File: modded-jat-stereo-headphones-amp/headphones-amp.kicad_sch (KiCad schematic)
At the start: 52 parts, among them J1 9V-15V, J2 9V-15V, J3 Input, J4 Headphones out, Q1 BD139, Q2 BD140, Q3 BD139, Q4 BD140, SW1 POWER ON, U1 NE5532

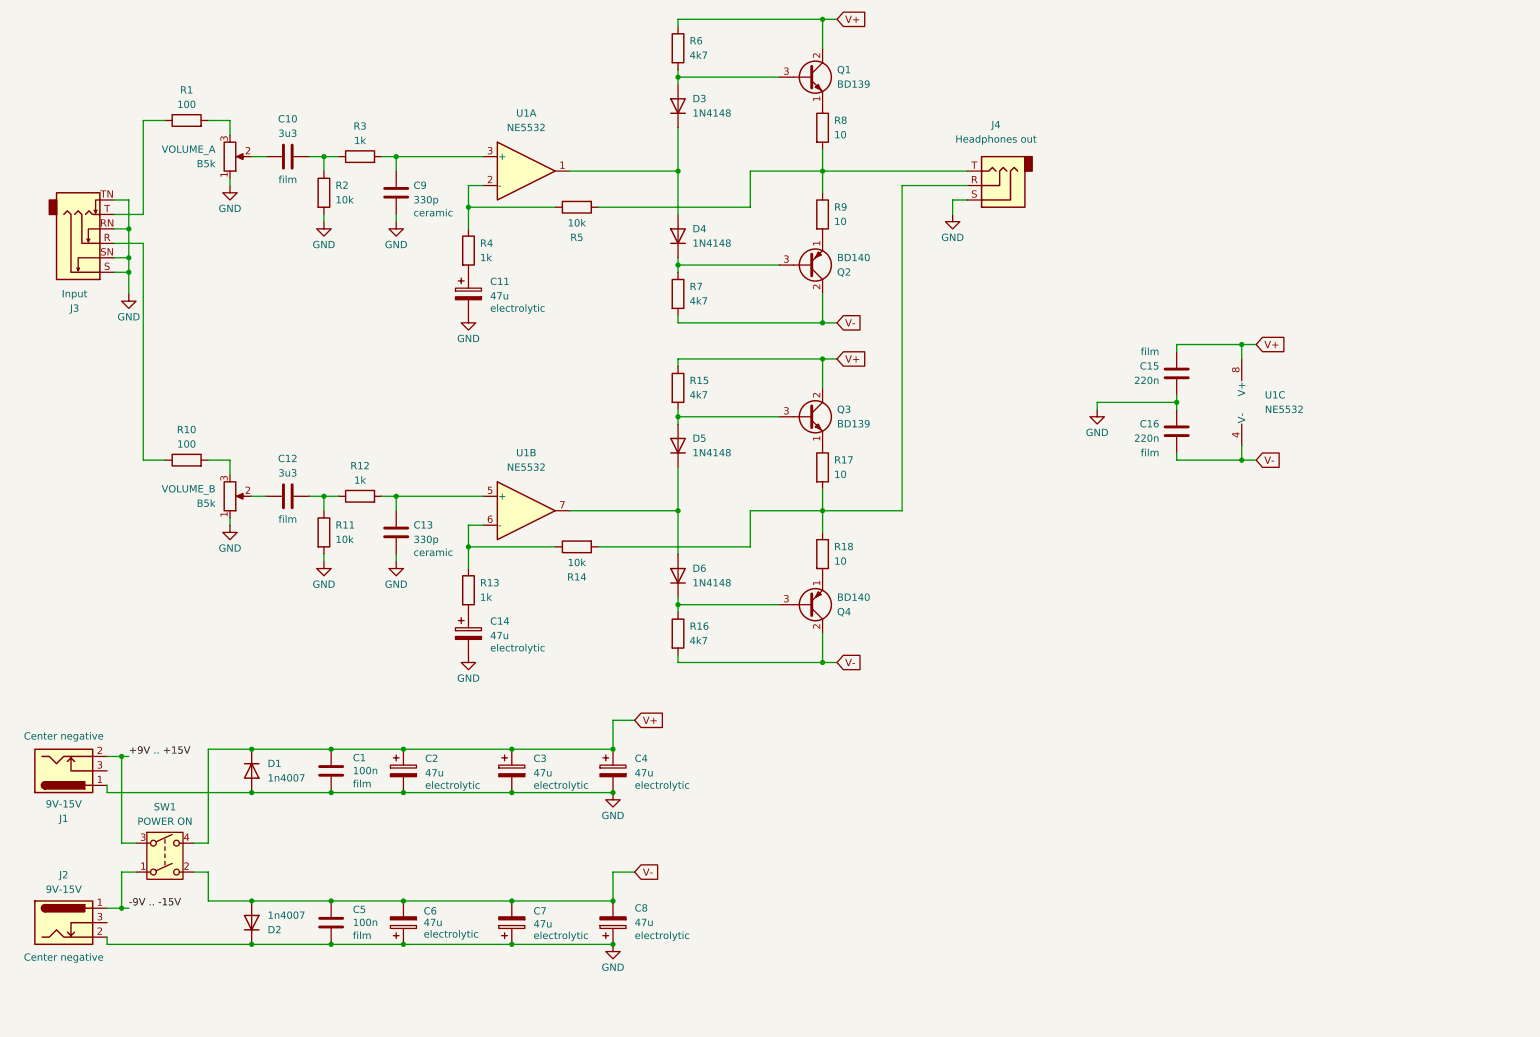
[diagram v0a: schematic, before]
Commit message: modded-jat-stereo-headphones-amp: r2-wip-1
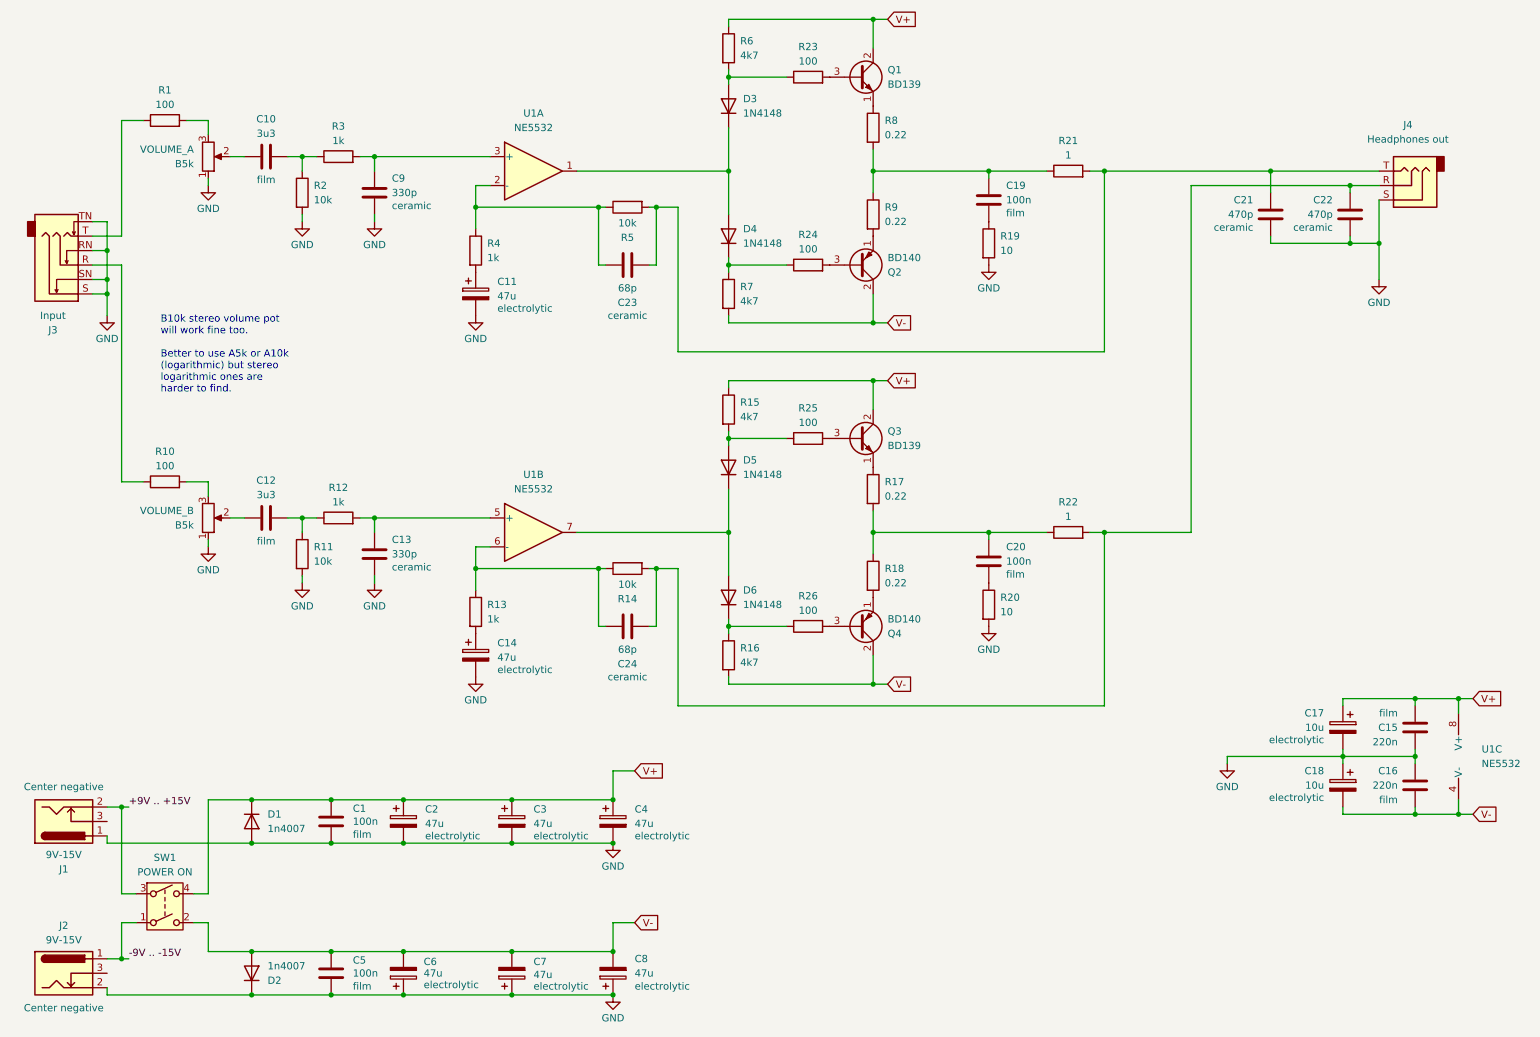
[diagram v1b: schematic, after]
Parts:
- added C17, C18: 10u, electrolytic, symbol Device:C_Polarized
- added C19, C20: 100n, symbol Device:C
- added C21, C22: 470p, symbol Device:C
- added C23, C24: 68p, symbol Device:C
- added R19, R20: 10, symbol Device:R
- added R21, R22: 1, symbol Device:R
- added R23, R24, R25, R26: 100, symbol Device:R
- R17, R18, R8, R9: value 10 -> 0.22
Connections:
- net GND: now also C17.2, C18.1, C21.2, C22.2, R19.2, R20.2
- net V+: now also C17.1
- net V-: now also C18.2
- net at D5.2 (A), R15.2: now also R25.1; no longer Q3.3 (B)
- net at D4.1 (K), R7.1: now also R24.1; no longer Q2.3 (B)
- net at R13.1, R14.1, U1.6 (-): now also C24.1
- net at D6.1 (K), R16.1: now also R26.1; no longer Q4.3 (B)
- net at D3.2 (A), R6.2: now also R23.1; no longer Q1.3 (B)
- net at R17.2, R18.1: now also C20.1, R22.1; no longer J4.R, R14.2
- net at R4.1, R5.1, U1.2 (-): now also C23.1
- net at R8.2, R9.1: now also C19.1, R21.1; no longer J4.T, R5.2
- new net: Q4.3 (B), R26.2
- new net: Q1.3 (B), R23.2
- new net: C19.2, R19.1
- new net: Q3.3 (B), R25.2
- new net: C22.1, C24.2, J4.R, R14.2, R22.2
- new net: C21.1, C23.2, J4.T, R21.2, R5.2
- new net: C20.2, R20.1
- new net: Q2.3 (B), R24.2
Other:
- note added: "B10k stereo volume pot will work fine too. Better to use A5k or A10k (logarithmic) but stereo logarithmic ones are harder to find."
- title: Headphones amp (modified “JAT Stereo Headphone Amp v1.0”) -> Wenzel’s Headphones Stereo Amp (dual supply)
- moved on the sheet: C1, C10, C11, C12, C13, C14, C15, C16, C2, C3, C4, C5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
